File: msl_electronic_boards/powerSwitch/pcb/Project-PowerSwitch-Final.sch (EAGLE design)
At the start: 130 parts, among them IC10 BTS6133, IC11 BTS6133, IC12 BTS6133, IC15 BTS6133, IC3 LM2574M-5.0, IC4 BTS555E3146, IC7 MAX202, Q1 16Mhz, T1 BC847, T2 BC849, T5 BC849, T6 BC849, T7 BC849

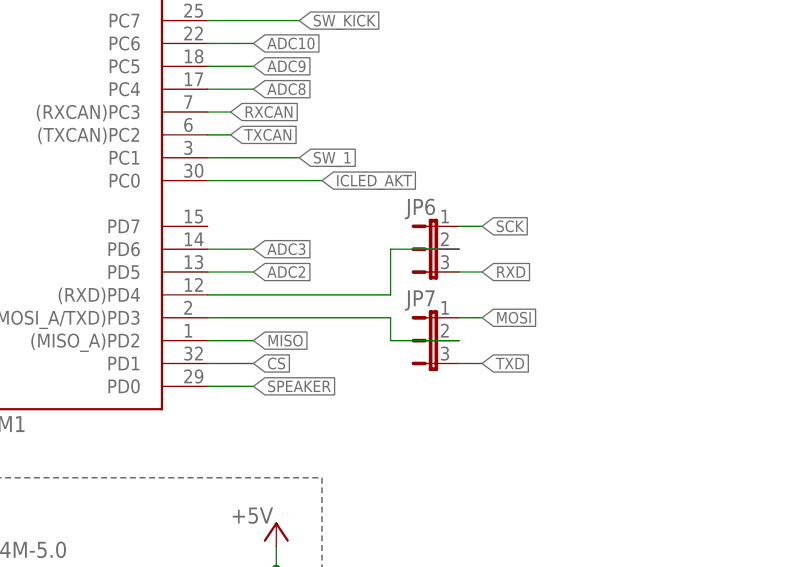
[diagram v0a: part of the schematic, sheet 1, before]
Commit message: PCB PowerSwitch
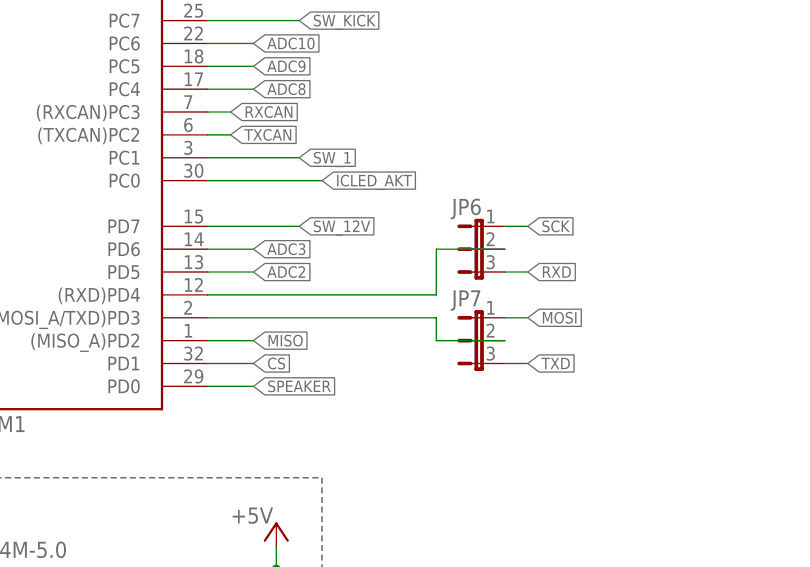
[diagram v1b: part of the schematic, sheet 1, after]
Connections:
- net SW_12V: now also U$2.PD7
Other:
- moved on the sheet: JP6, JP7
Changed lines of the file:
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@@
 <attribute name="VALUE" x="0" y="160.02" size="1.778" layer="96"/>
 </instance>
-<instance part="JP6" gate="1" x="121.92" y="109.22" rot="MR270"/>
-<instance part="JP7" gate="1" x="121.92" y="99.06" rot="MR270"/>
+<instance part="JP6" gate="1" x="127" y="109.22" rot="MR270"/>
+<instance part="JP7" gate="1" x="127" y="99.06" rot="MR270"/>
 <instance part="SV4" gate="G$1" x="233.68" y="114.3"/>
 <instance part="P+7" gate="1" x="220.98" y="121.92" smashed="yes">
@@
 <net name="TXD" class="0">
 <segment>
-<wire x1="124.46" y1="96.52" x2="127" y2="96.52" width="0.1524" layer="91"/>
-<label x="127" y="96.52" size="1.27" layer="95" xref="yes"/>
+<wire x1="129.54" y1="96.52" x2="132.08" y2="96.52" width="0.1524" layer="91"/>
+<label x="132.08" y="96.52" size="1.27" layer="95" xref="yes"/>
 <pinref part="JP7" gate="1" pin="3"/>
 </segment>
@@
 <net name="RXD" class="0">
 <segment>
-<wire x1="124.46" y1="106.68" x2="127" y2="106.68" width="0.1524" layer="91"/>
-<label x="127" y="106.68" size="1.27" layer="95" xref="yes"/>
+<wire x1="129.54" y1="106.68" x2="132.08" y2="106.68" width="0.1524" layer="91"/>
+<label x="132.08" y="106.68" size="1.27" layer="95" xref="yes"/>
 <pinref part="JP6" gate="1" pin="3"/>
 </segment>
@@
 <net name="SCK" class="0">
 <segment>
-<label x="127" y="111.76" size="1.27" layer="95" xref="yes"/>
-<wire x1="124.46" y1="111.76" x2="127" y2="111.76" width="0.1524" layer="91"/>
+<label x="132.08" y="111.76" size="1.27" layer="95" xref="yes"/>
+<wire x1="129.54" y1="111.76" x2="132.08" y2="111.76" width="0.1524" layer="91"/>
 <pinref part="JP6" gate="1" pin="1"/>
 </segment>
@@
 <net name="MOSI" class="0">
 <segment>
-<label x="127" y="101.6" size="1.27" layer="95" xref="yes"/>
-<wire x1="124.46" y1="101.6" x2="127" y2="101.6" width="0.1524" layer="91"/>
+<label x="132.08" y="101.6" size="1.27" layer="95" xref="yes"/>
+<wire x1="129.54" y1="101.6" x2="132.08" y2="101.6" width="0.1524" layer="91"/>
 <pinref part="JP7" gate="1" pin="1"/>
 </segment>
@@
 <label x="223.52" y="134.62" size="1.27" layer="95" rot="R180" xref="yes"/>
 <pinref part="SV2" gate="G$1" pin="4"/>
+</segment>
+<segment>
+<wire x1="96.52" y1="111.76" x2="106.68" y2="111.76" width="0.1524" layer="91"/>
+<label x="106.68" y="111.76" size="1.27" layer="95" xref="yes"/>
+<pinref part="U$2" gate="G$1" pin="PD7"/>
 </segment>
 </net>
@@
 <pinref part="JP6" gate="1" pin="2"/>
 <pinref part="U$2" gate="G$1" pin="(RXD)PD4"/>
-<wire x1="124.46" y1="109.22" x2="116.84" y2="109.22" width="0.1524" layer="91"/>
-<wire x1="116.84" y1="109.22" x2="116.84" y2="104.14" width="0.1524" layer="91"/>
-<wire x1="116.84" y1="104.14" x2="96.52" y2="104.14" width="0.1524" layer="91"/>
+<wire x1="129.54" y1="109.22" x2="121.92" y2="109.22" width="0.1524" layer="91"/>
+<wire x1="121.92" y1="109.22" x2="121.92" y2="104.14" width="0.1524" layer="91"/>
+<wire x1="121.92" y1="104.14" x2="96.52" y2="104.14" width="0.1524" layer="91"/>
 </segment>
 </net>
@@
 <segment>
 <pinref part="JP7" gate="1" pin="2"/>
-<wire x1="124.46" y1="99.06" x2="116.84" y2="99.06" width="0.1524" layer="91"/>
-<wire x1="116.84" y1="99.06" x2="116.84" y2="101.6" width="0.1524" layer="91"/>
+<wire x1="129.54" y1="99.06" x2="121.92" y2="99.06" width="0.1524" layer="91"/>
+<wire x1="121.92" y1="99.06" x2="121.92" y2="101.6" width="0.1524" layer="91"/>
 <pinref part="U$2" gate="G$1" pin="(MOSI_A/TXD)PD3"/>
-<wire x1="116.84" y1="101.6" x2="96.52" y2="101.6" width="0.1524" layer="91"/>
-</segment>
-</net>
+<wire x1="121.92" y1="101.6" x2="96.52" y2="101.6" width="0.1524" layer="91"/>
+</segment>
+</net>
